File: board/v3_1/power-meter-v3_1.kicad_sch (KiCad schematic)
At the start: 50 parts, among them J1 Screw_Terminal_01x04, J2 Screw_Terminal_01x02, J4 Conn_01x03, J5 Conn_01x02_Pin, U1 ADM2486, U2 FM24C64B, U3 INA228, U4 ATtiny1624-SS, U5 L78L05_TO92, U7 L78L05_TO92

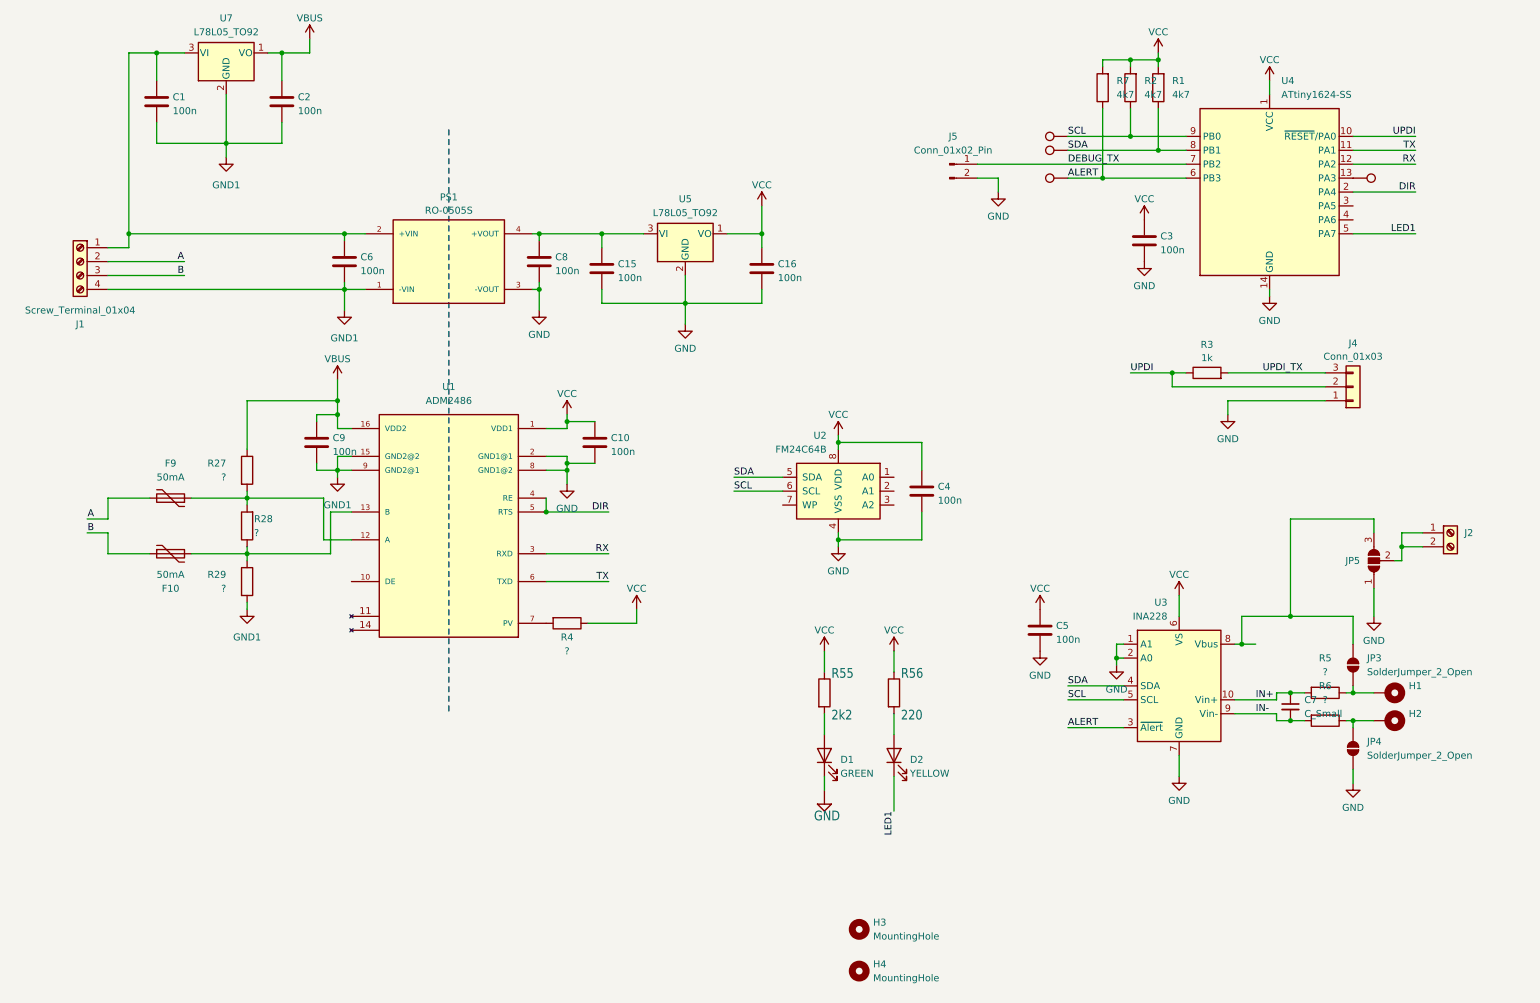
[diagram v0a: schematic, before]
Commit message: minor schematic updates
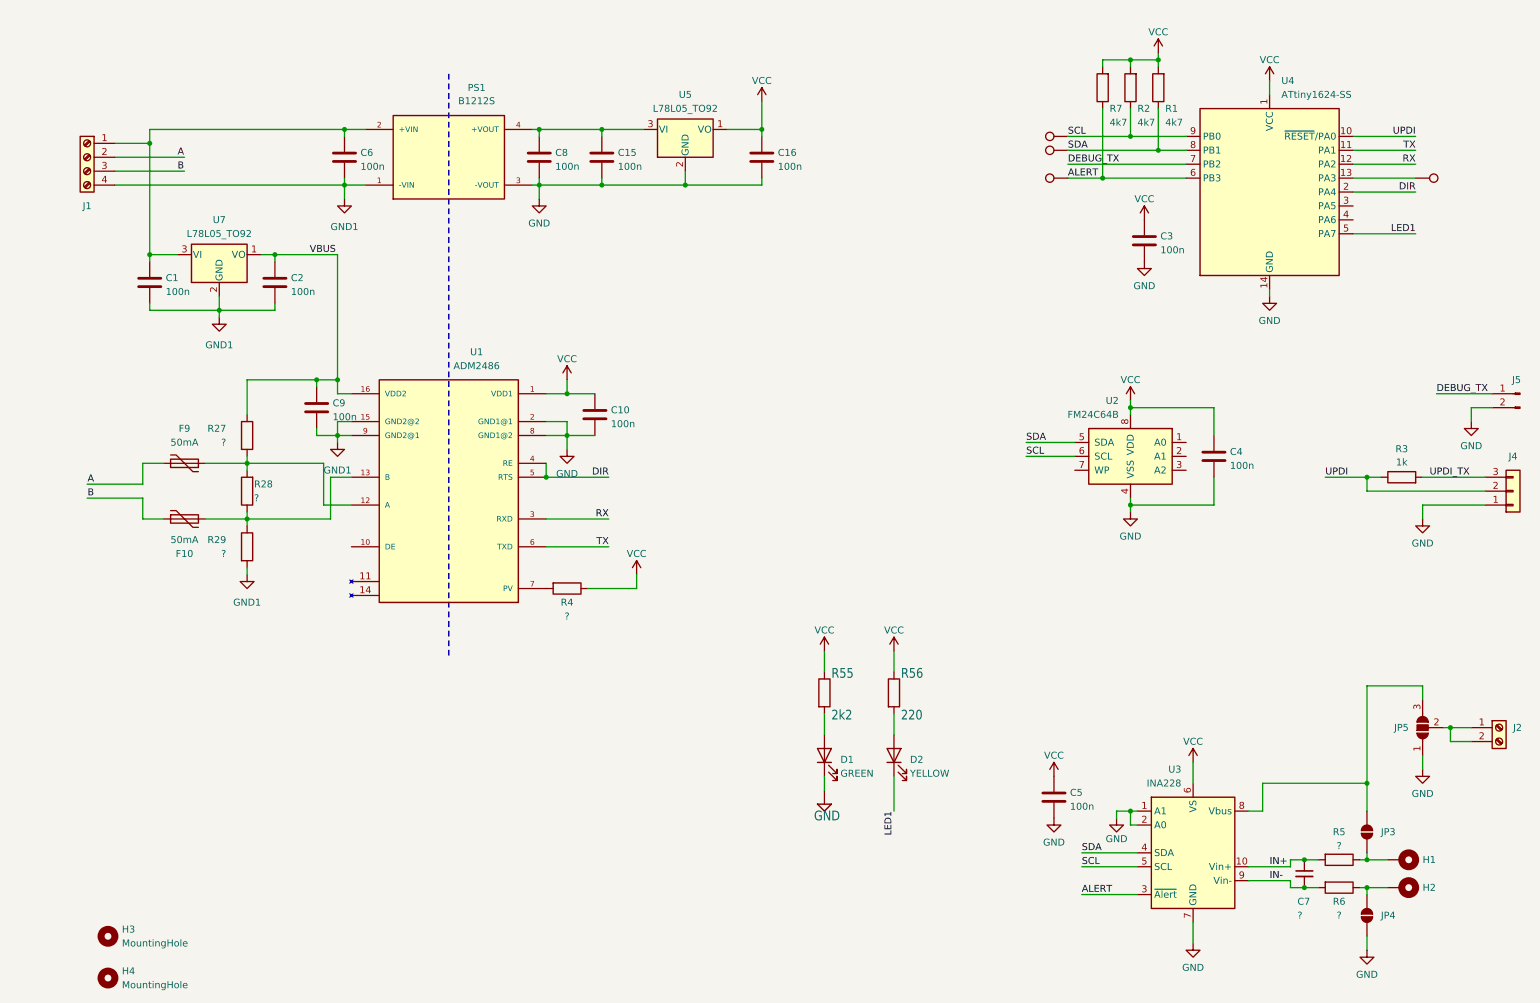
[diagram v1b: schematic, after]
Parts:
- C7: value C_Small -> ?
- PS1: value RO-0505S -> B1212S
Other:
- moved on the sheet: C1, C10, C15, C16, C2, C4, C5, C6, C7, C8, C9, F10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
